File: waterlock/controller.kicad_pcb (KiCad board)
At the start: 2 copper layers, 78.7 x 50.9 mm, 28 parts, among them CON1 AVR-ISP-10, J1 v5, J2 v12, J3 m1, J4 m2, J5 Battery, J6 L1, J7 L2, SW1 Turn, U1 ATMEGA8-16PU, U3 L293D

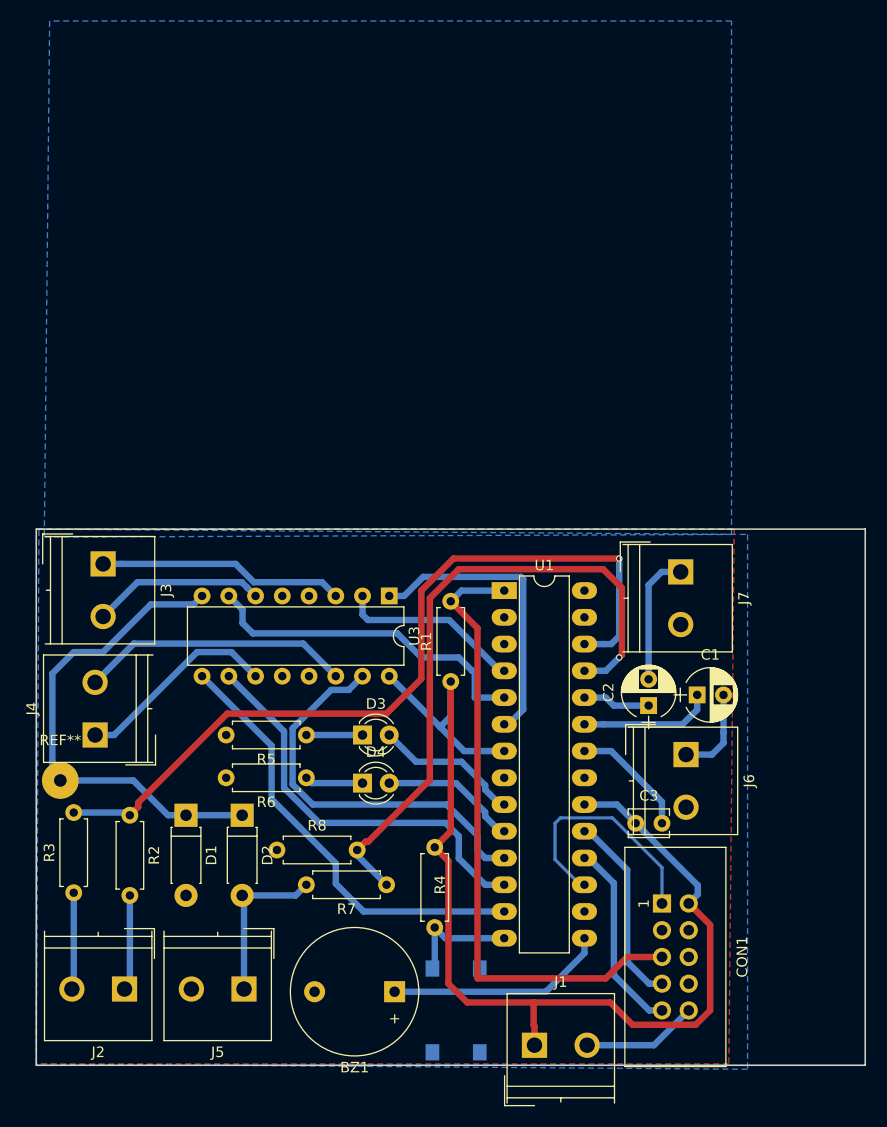
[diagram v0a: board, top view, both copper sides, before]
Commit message: firmware start
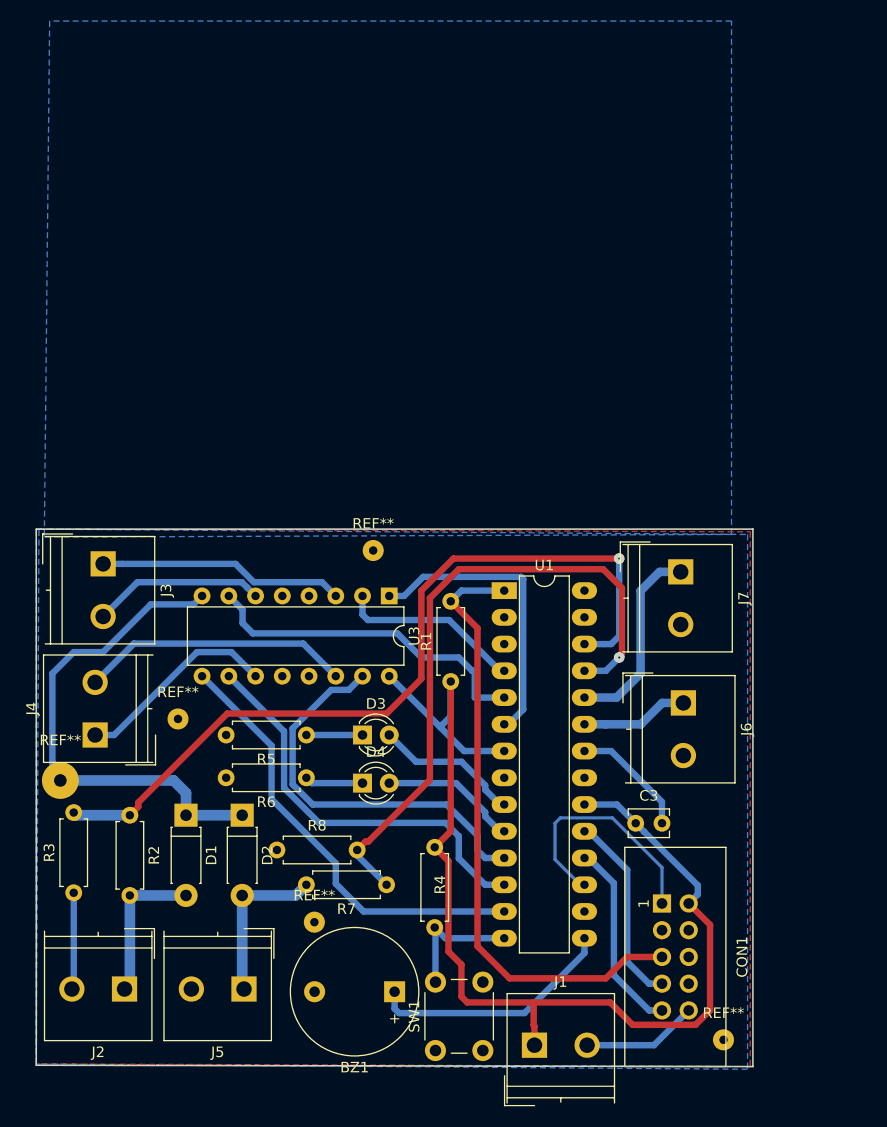
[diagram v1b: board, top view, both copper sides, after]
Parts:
- removed C1, C2: 10mF, Capacitors_THT:CP_Radial_D5.0mm_P2.50mm
- added REF**: , Wire_Pads:SolderWirePad_single_0-8mmDrill, F.Cu at (25.4, 30.2)
- added REF**: , Wire_Pads:SolderWirePad_single_0-8mmDrill, F.Cu at (38.4, 49.5)
- added REF**: , Wire_Pads:SolderWirePad_single_0-8mmDrill, F.Cu at (77.2, 60.7)
- added REF**: , Wire_Pads:SolderWirePad_single_0-8mmDrill, F.Cu at (43.9, 14.2)
- REF**: value SolderWirePad_single_1-2mmDrill -> (none)
- SW1: footprint Buttons_Switches_SMD:SW_SPST_PTS645 -> Buttons_Switches_THT:SW_PUSH_6mm_h8.5mm; moved to F.Cu
- moved J6 4.91 mm to (73.4, 28.7)
- moved SW1 4.28 mm to (49.9, 61.7), turned to 90 degrees
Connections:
- J6 pad 1: Net-(C1-Pad2) -> /Line1
- J7 pad 1: Net-(C2-Pad2) -> /Line2
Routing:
- net Net-(C2-Pad2): track 12.5 -> 0.00 mm
- net /Line2: track 6.41 -> 18.7 mm
- net Net-(C1-Pad2): track 8.58 -> 0.00 mm
- net /acdc_pwr: track 9.10 -> 14.4 mm
- net /buzz: track 21.0 -> 23.6 mm
- net /Line1: track 12.7 -> 10.2 mm
- net /RESET: track 60.7 -> 58.9 mm
- net +12V: track 46.4 -> 47.6 mm
- net /btn_1: track 11.0 -> 12.2 mm
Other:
- board size 78.7 x 50.9 mm -> 68.1 x 51.1 mm
- rule via_min_drill: 0.3 -> 0.1524
- rule via_min_size: 0.4 -> 0.1524
